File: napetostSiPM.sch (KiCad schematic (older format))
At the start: 24 parts, among them U1 AD8001AN, U2 MAX5026, U3 INA168, U4 AD8001AN, U5 LM7705

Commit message: Add files via upload
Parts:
- removed C1, C10, C2, C3, C4, C5, C6, C7, C8, C9: C, Capacitor_SMD:C_0805_2012Metric_Pad1.15x1.40mm_HandSolder, symbol Device:C
- removed D1: D_Schottky, symbol Device:D_Schottky
- removed L1: L, symbol Device:L
- removed R1, R2, R3, R4, R5, R6, R7: R, Resistor_SMD:R_0805_2012Metric_Pad1.15x1.40mm_HandSolder, symbol Device:R
- removed U1, U4: AD8001AN, Package_DIP:DIP-8_W7.62mm, symbol Amplifier_Operational:AD8001AN
- removed U2: MAX5026, MAX5026footprint:SOT95P280X145-6N, symbol Amplifier_Difference:MAX5026
- removed U3: INA168, Package_TO_SOT_SMD:SOT-23-5, symbol Amplifier_Current:INA168
- removed U5: LM7705, LM7705footprint:SOP65P490X110-8N, symbol Amplifier_Difference:LM7705
- added J1: Conn_01x14_Male, symbol Connector:Conn_01x14_Male
- added J2: Conn_ARM_JTAG_SWD_10, Connector_PinHeader_1.27mm:PinHeader_2x05_P1.27mm_Vertical_SMD, symbol Connector:Conn_ARM_JTAG_SWD_10
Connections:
- net labels added: +3.3V, ANALOG, BIAS, BRANJE, DIGITAL, NRST, SCL, SDA, SWDCLK, SWDIO, SWO
- net labels removed: GNDboljse, MAX:32V
- wire segments 97 -> 18
- no-connect marks 0 -> 1

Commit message: Add files via upload
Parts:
- removed J1: Conn_01x14_Male, symbol Connector:Conn_01x14_Male
- added J1: Conn_01x13_Male, symbol Connector:Conn_01x13_Male
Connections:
- net labels added: NTC
- wire segments 18 -> 17
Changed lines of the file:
@@
 Wire Wire Line
 	8800 2650 8250 2650
-Text GLabel 8800 2750 2    50   Input ~ 0
+Text GLabel 8800 2550 2    50   Input ~ 0
 SCL
-Text GLabel 8800 2850 2    50   Input ~ 0
+Text GLabel 8800 2650 2    50   Input ~ 0
 SDA
 Wire Wire Line
@@
 SWO
 $Comp
-L Connector:Conn_01x14_Male J1
-U 1 1 61F59C6C
+L Connector:Conn_01x13_Male J1
+U 1 1 61EE8518
 P 8050 2150
 F 0 "J1" H 8156 2928 50  0000 C CNN
-F 1 "Conn_01x14_Male" H 8156 2837 50  0000 C CNN
+F 1 "Conn_01x13_Male" H 8156 2837 50  0000 C CNN
 F 2 "" H 8050 2150 50  0001 C CNN
 F 3 "~" H 8050 2150 50  0001 C CNN
@@
 $EndComp
 Wire Wire Line
-	8250 2750 8800 2750
-Wire Wire Line
-	8250 2850 8800 2850
-$Comp
-L power:+3.3V #PWR0101
-U 1 1 61F5A467
-P 8800 2550
-F 0 "#PWR0101" H 8800 2400 50  0001 C CNN
-F 1 "+3.3V" V 8815 2678 50  0000 L CNN
-F 2 "" H 8800 2550 50  0001 C CNN
-F 3 "" H 8800 2550 50  0001 C CNN
-	1    8800 2550
-	0    1    1    0
-$EndComp
-$Comp
-L power:GND #PWR0102
-U 1 1 61F5A61E
-P 8800 2650
-F 0 "#PWR0102" H 8800 2400 50  0001 C CNN
-F 1 "GND" V 8805 2522 50  0000 R CNN
-F 2 "" H 8800 2650 50  0001 C CNN
-F 3 "" H 8800 2650 50  0001 C CNN
-	1    8800 2650
-	0    -1   -1   0
-$EndComp
+	8600 2750 8250 2750
+Text GLabel 8600 2750 2    50   Input ~ 0
+NTC
 $EndSCHEMATC

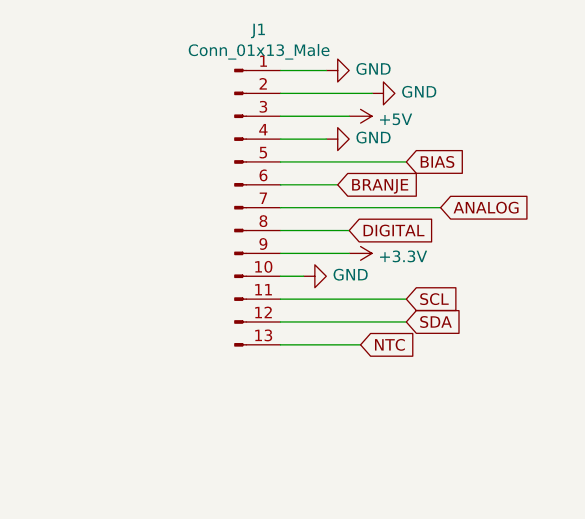
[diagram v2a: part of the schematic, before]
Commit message: Add files via upload
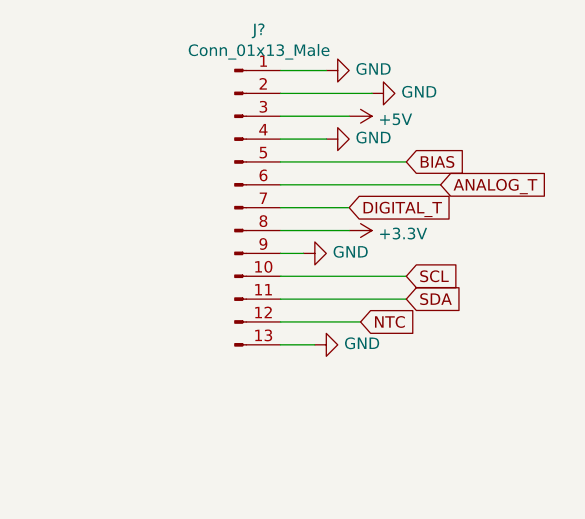
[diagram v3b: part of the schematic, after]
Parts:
- removed J1: Conn_01x13_Male, symbol Connector:Conn_01x13_Male
- added J?: Conn_01x13_Male, symbol Connector:Conn_01x13_Male
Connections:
- net +3V3: now also J?.8 (Pin_8)
- net +5V: now also J?.3 (Pin_3)
- net BIAS: now also J?.5 (Pin_5)
- net GND: now also J?.1 (Pin_1), J?.13 (Pin_13), J?.2 (Pin_2), J?.4 (Pin_4), J?.9 (Pin_9)
- net NTC: now also J?.12 (Pin_12)
- net SCL: now also J?.10 (Pin_10)
- net SDA: now also J?.11 (Pin_11)
- new net ANALOG_T: J?.6 (Pin_6)
- new net DIGITAL_T: J?.7 (Pin_7)
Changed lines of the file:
@@
 	8800 1950 8250 1950
 Wire Wire Line
-	8500 2050 8250 2050
+	8950 2050 8250 2050
 Wire Wire Line
-	8950 2150 8250 2150
-Text GLabel 8950 2150 2    50   Input ~ 0
-ANALOG
-Wire Wire Line
-	8550 2350 8250 2350
+	8550 2250 8250 2250
 $Comp
 L power:+3.3V #PWR06
 U 1 1 61EC92B3
-P 8550 2350
-F 0 "#PWR06" H 8550 2200 50  0001 C CNN
-F 1 "+3.3V" V 8565 2478 50  0000 L CNN
-F 2 "" H 8550 2350 50  0001 C CNN
-F 3 "" H 8550 2350 50  0001 C CNN
-	1    8550 2350
+P 8550 2250
+F 0 "#PWR06" H 8550 2100 50  0001 C CNN
+F 1 "+3.3V" V 8565 2378 50  0000 L CNN
+F 2 "" H 8550 2250 50  0001 C CNN
+F 3 "" H 8550 2250 50  0001 C CNN
+	1    8550 2250
 	0    1    1    0
 $EndComp
 Wire Wire Line
-	8350 2450 8250 2450
+	8350 2350 8250 2350
 $Comp
 L power:GND #PWR01
 U 1 1 61ED4863
-P 8350 2450
-F 0 "#PWR01" H 8350 2200 50  0001 C CNN
-F 1 "GND" V 8355 2322 50  0000 R CNN
-F 2 "" H 8350 2450 50  0001 C CNN
-F 3 "" H 8350 2450 50  0001 C CNN
-	1    8350 2450
+P 8350 2350
+F 0 "#PWR01" H 8350 2100 50  0001 C CNN
+F 1 "GND" V 8355 2222 50  0000 R CNN
+F 2 "" H 8350 2350 50  0001 C CNN
+F 3 "" H 8350 2350 50  0001 C CNN
+	1    8350 2350
 	0    -1   -1   0
 $EndComp
 Wire Wire Line
+	8800 2450 8250 2450
+Wire Wire Line
 	8800 2550 8250 2550
-Wire Wire Line
-	8800 2650 8250 2650
+Text GLabel 8800 2450 2    50   Input ~ 0
+SCL
 Text GLabel 8800 2550 2    50   Input ~ 0
-SCL
-Text GLabel 8800 2650 2    50   Input ~ 0
 SDA
 Wire Wire Line
-	8550 2250 8250 2250
-Text GLabel 8550 2250 2    50   Input ~ 0
-DIGITAL
+	8550 2150 8250 2150
 $Comp
 L Connector:Conn_ARM_JTAG_SWD_10 J?
@@
 Text GLabel 8800 1950 2    50   Input ~ 0
 BIAS
-Text GLabel 8500 2050 2    50   Input ~ 0
-BRANJE
 Text GLabel 9050 4300 2    50   Input ~ 0
 NRST
@@
 Text GLabel 9050 4700 2    50   Input ~ 0
 SWO
+Wire Wire Line
+	8600 2650 8250 2650
+Text GLabel 8600 2650 2    50   Input ~ 0
+NTC
+Wire Wire Line
+	8400 2750 8250 2750
 $Comp
-L Connector:Conn_01x13_Male J1
-U 1 1 61EE8518
+L power:GND #PWR0103
+U 1 1 61EFC12A
+P 8400 2750
+F 0 "#PWR0103" H 8400 2500 50  0001 C CNN
+F 1 "GND" V 8405 2622 50  0000 R CNN
+F 2 "" H 8400 2750 50  0001 C CNN
+F 3 "" H 8400 2750 50  0001 C CNN
+	1    8400 2750
+	0    -1   -1   0
+$EndComp
+$Comp
+L Connector:Conn_01x13_Male J?
+U 1 1 61F8017B
 P 8050 2150
-F 0 "J1" H 8156 2928 50  0000 C CNN
+F 0 "J?" H 8156 2928 50  0000 C CNN
 F 1 "Conn_01x13_Male" H 8156 2837 50  0000 C CNN
 F 2 "" H 8050 2150 50  0001 C CNN
@@
 	1    0    0    -1
 $EndComp
-Wire Wire Line
-	8600 2750 8250 2750
-Text GLabel 8600 2750 2    50   Input ~ 0
-NTC
+Text GLabel 8950 2050 2    50   Input ~ 0
+ANALOG_T
+Text GLabel 8550 2150 2    50   Input ~ 0
+DIGITAL_T
 $EndSCHEMATC

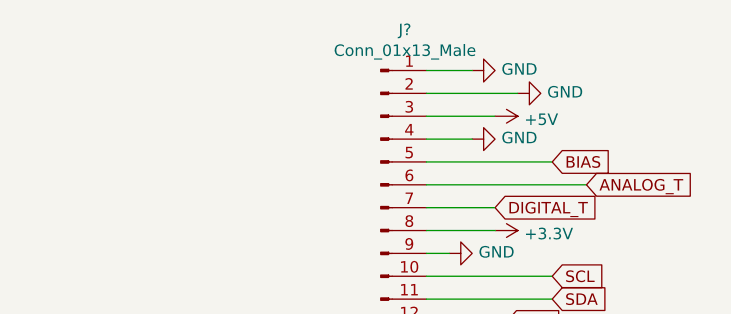
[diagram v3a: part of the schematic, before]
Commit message: Add files via upload
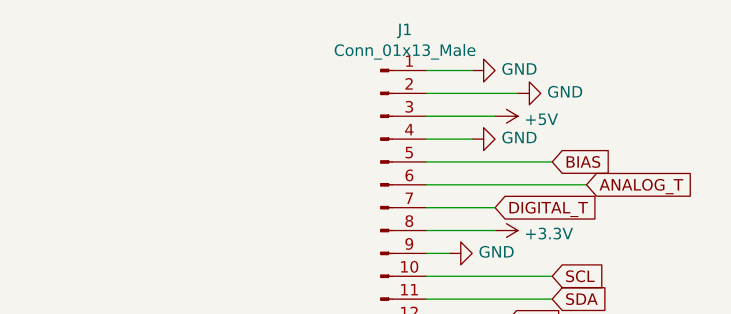
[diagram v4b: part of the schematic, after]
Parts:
- J1: renamed from J?; footprint (none) -> Connector_PinHeader_2.54mm:PinHeader_1x13_P2.54mm_Vertical
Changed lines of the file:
@@
 $EndComp
 $Comp
-L Connector:Conn_01x13_Male J?
+L Connector:Conn_01x13_Male J1
 U 1 1 61F8017B
 P 8050 2150
-F 0 "J?" H 8156 2928 50  0000 C CNN
+F 0 "J1" H 8156 2928 50  0000 C CNN
 F 1 "Conn_01x13_Male" H 8156 2837 50  0000 C CNN
-F 2 "" H 8050 2150 50  0001 C CNN
+F 2 "Connector_PinHeader_2.54mm:PinHeader_1x13_P2.54mm_Vertical" H 8050 2150 50  0001 C CNN
 F 3 "~" H 8050 2150 50  0001 C CNN
 	1    8050 2150
